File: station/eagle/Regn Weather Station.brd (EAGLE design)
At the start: 64.1 x 48.6 mm, 6 parts

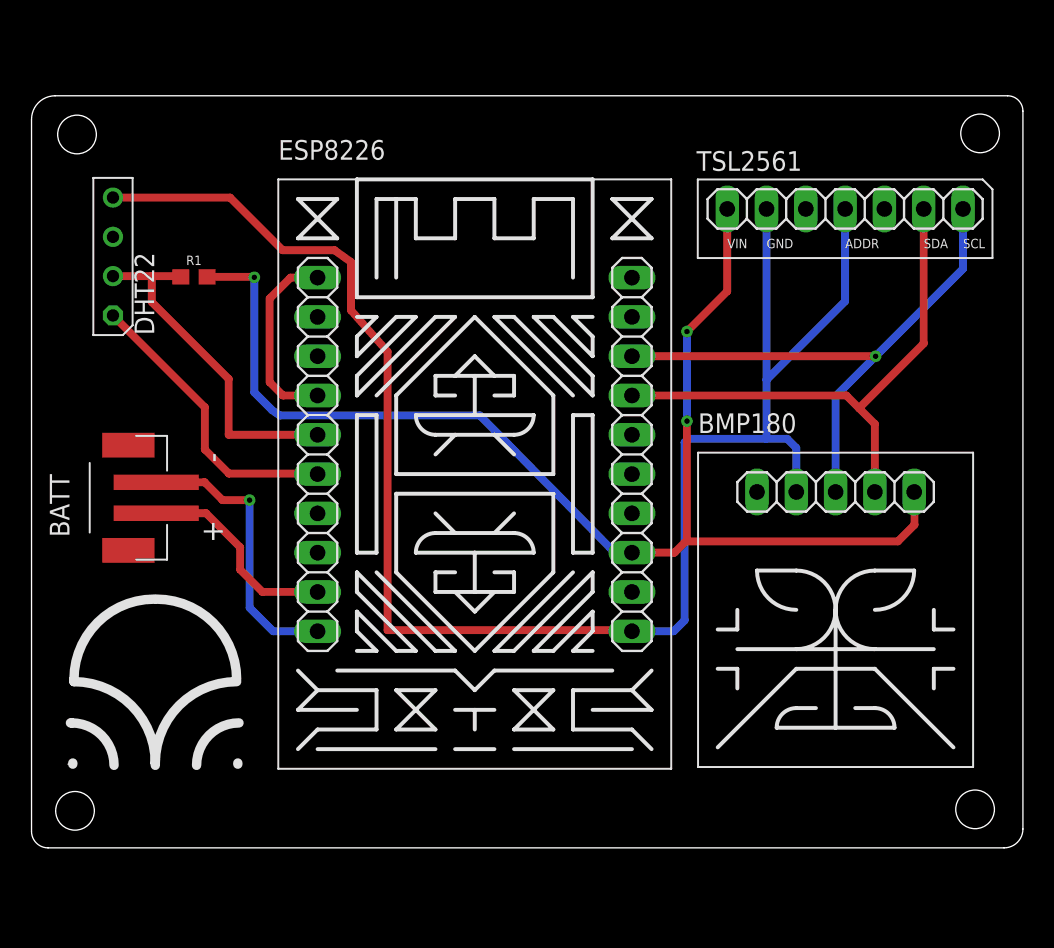
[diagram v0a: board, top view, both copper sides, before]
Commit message: PCB optimizations and refining
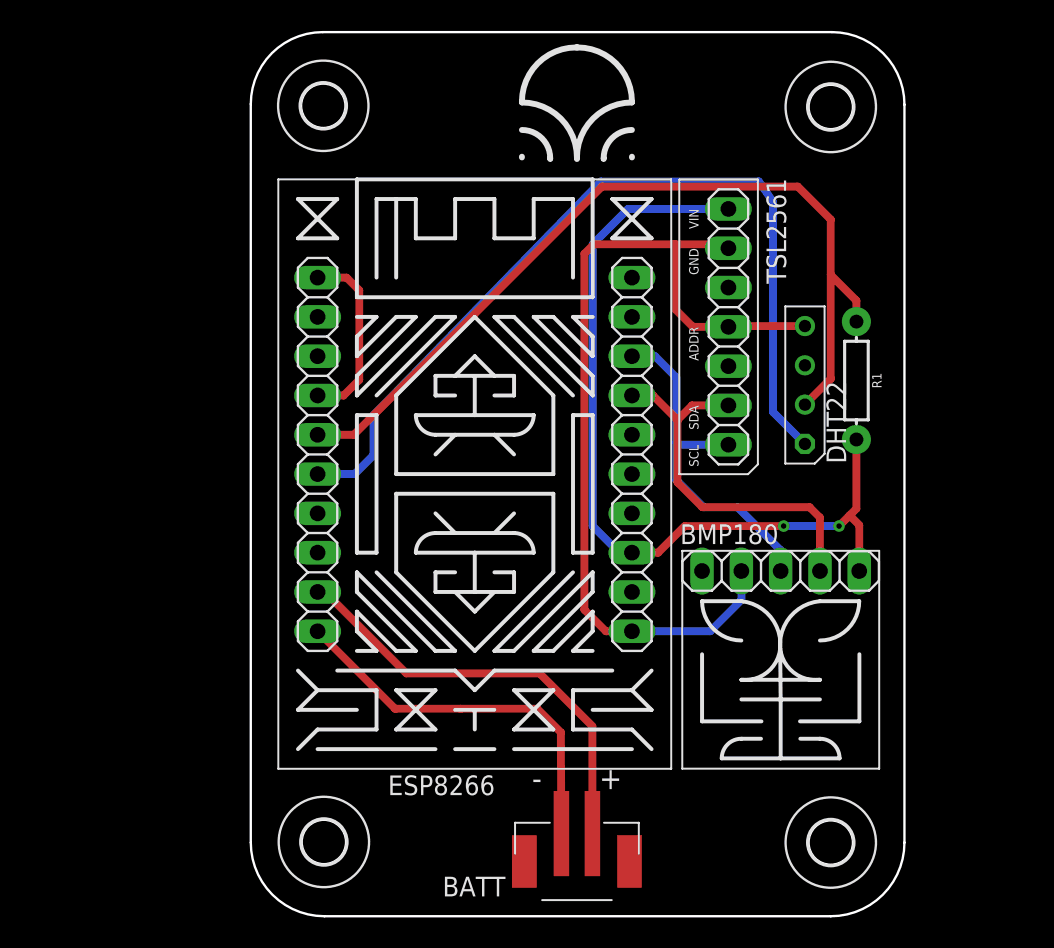
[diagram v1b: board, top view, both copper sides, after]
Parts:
- added U$1, U$2, U$3, U$4: (no value), holes:2,8
- R1: device SparkFun-Resistors:0603 -> SparkFun-Resistors:AXIAL-0.3
- moved DHT22 45.5 mm to (51.7, 61.2)
- moved R1 43.3 mm to (55.0, 61.5), turned to 270 degrees
- moved BATT 37.3 mm to (36.9, 30.4), turned to 180 degrees
- moved TSL2561 10.7 mm to (46.7, 65.0), turned to 270 degrees
- moved BMP180 10.7 mm to (43.7, 50.6)
- renumbered ESP8226 to ESP8266
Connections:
- net 3.3V: now also R1.P$2; no longer R1.2
- net N$1: now also R1.P$1; no longer R1.1
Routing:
- net GND: track 111.4 -> 59.5 mm
- net N$2: track 19.1 -> 56.1 mm
- net N$1: track 22.5 -> 57.1 mm
- net 3.3V: track 83.0 -> 55.2 mm, vias 3 -> 2
- net N$6: track 13.4 -> 28.3 mm
- net N$5: track 37.5 -> 23.5 mm, vias 1 -> 0
- net N$3: track 35.5 -> 24.9 mm
- net N$7: track 18.5 -> 25.0 mm, vias 1 -> 0
- net N$4: track 12.5 -> 11.9 mm
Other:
- board size 64.1 x 48.6 mm -> 42.3 x 57.1 mm
- board text added: "Regn 0.1 6 Blóstm 226 [ Autophagy ]"
